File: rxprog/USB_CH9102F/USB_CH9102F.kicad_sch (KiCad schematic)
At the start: 26 parts, among them J1 5077CR-16-SMC2-BK-TR, J2 USB/OPT, J3 Serial In/Out Full, J4 GPIO, J5 SUSPEND, J6 /SUSPEND, J7 /ACT, J8 /RST, J9 Serial In/Out, SW1 3P-SW, U1 CH9102F, U2 NJU7223DL1-33

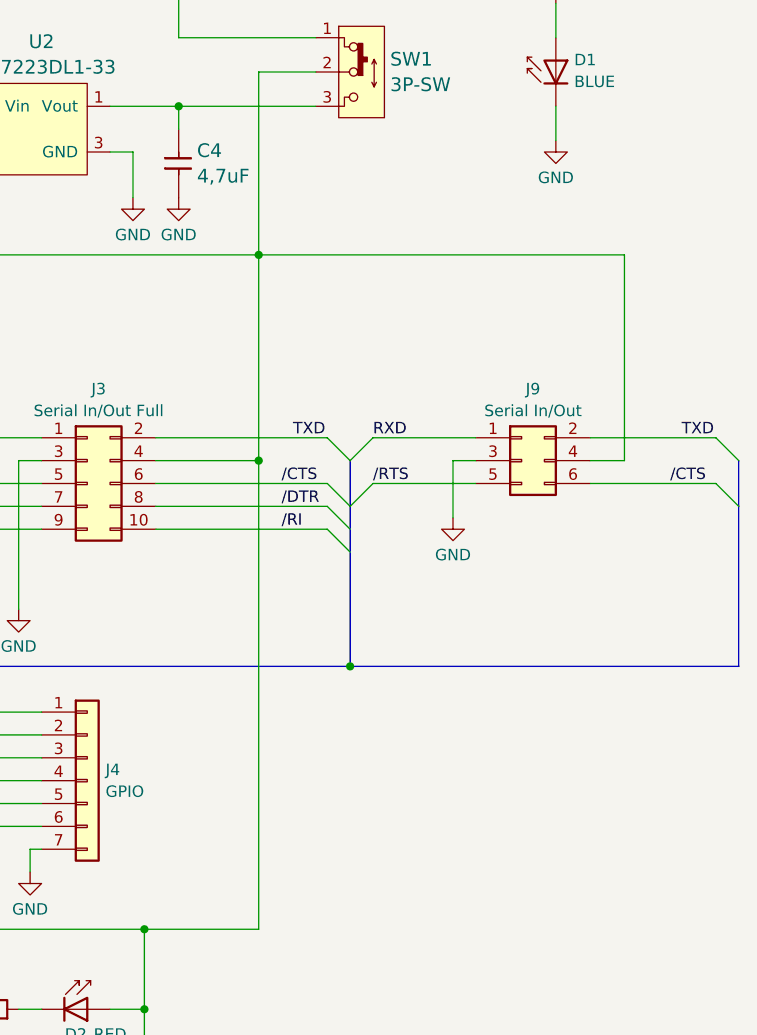
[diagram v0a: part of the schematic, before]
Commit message: Update: sch/pcb
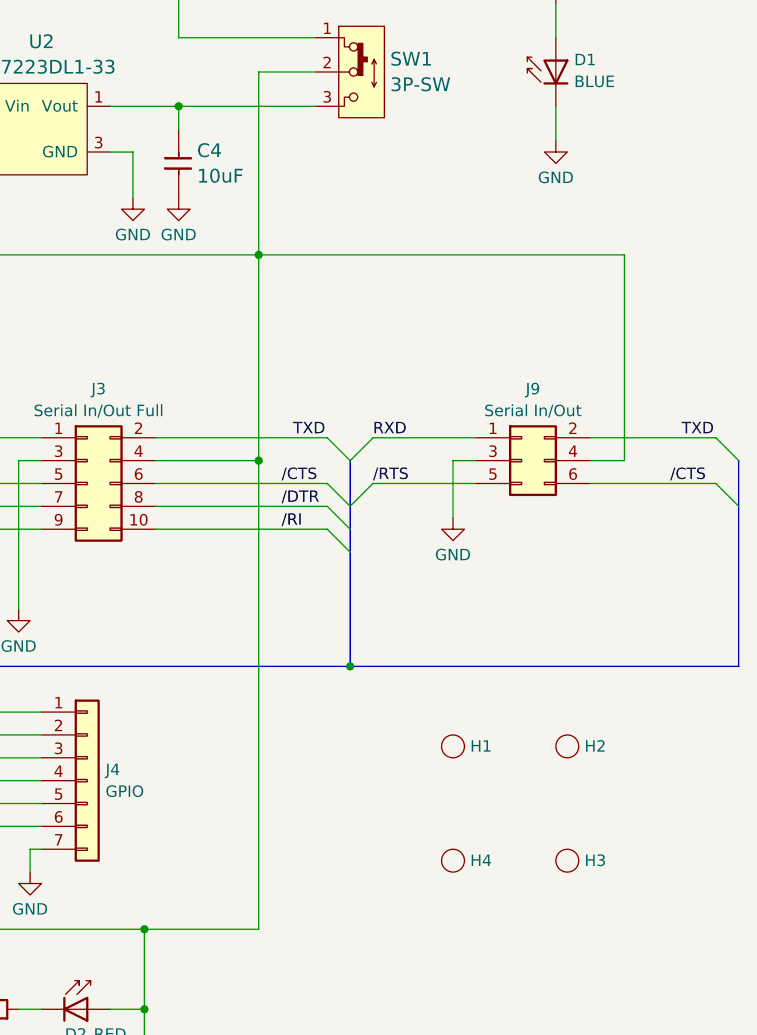
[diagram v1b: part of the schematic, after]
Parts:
- added H1, H2, H3, H4: (no value), KiCAD_lib:Hole3.2mm, symbol analog:HOLE
- C4: value 4,7uF -> 10uF
